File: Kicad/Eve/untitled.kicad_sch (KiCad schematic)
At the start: 9 parts

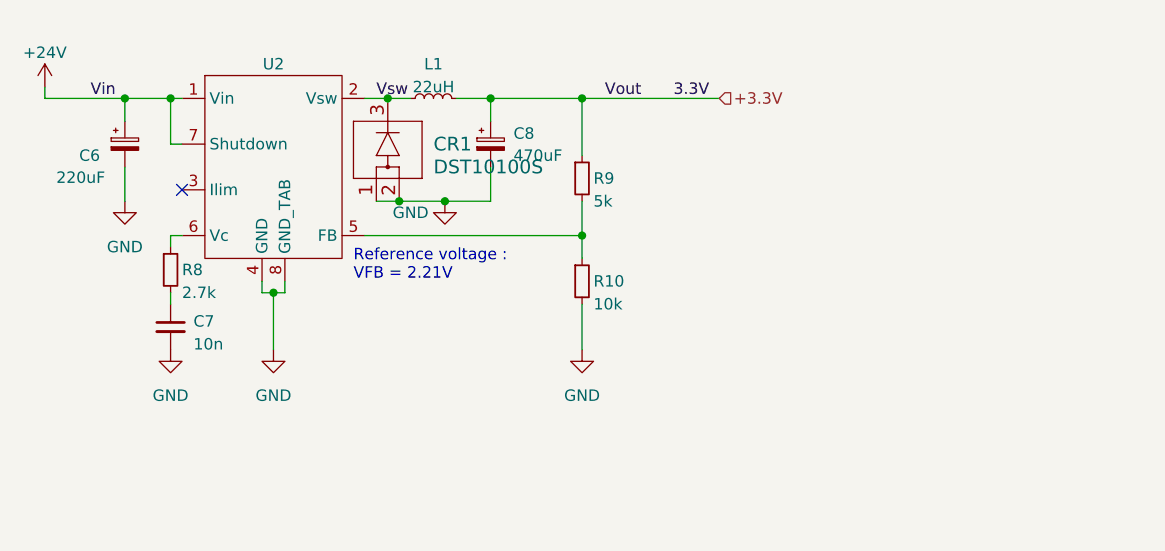
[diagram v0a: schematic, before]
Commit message: updtated Kicad ver 7.11.23
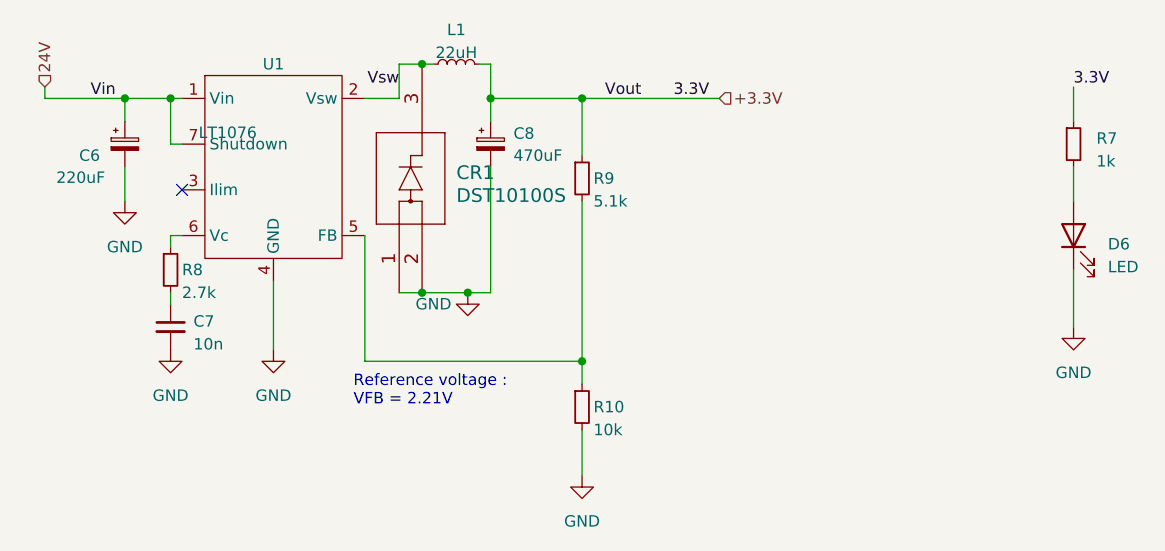
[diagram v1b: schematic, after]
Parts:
- removed U2: ~, libs:LT1076CR-PBF, symbol custom:LT1076
- added D6: LED, LED_SMD:LED_0603_1608Metric_Pad1.05x0.95mm_HandSolder, symbol Device:LED
- added R7: 1k, Resistor_SMD:R_0603_1608Metric_Pad0.98x0.95mm_HandSolder, symbol Device:R_Small
- added U1: LT1076, symbol custom:LT1076
- CR1: footprint libs:DST10100S -> TO277B_LTF
- R9: value 5k -> 5.1k
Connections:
- net +3.3V: now also R7.1
- net GND: now also D6.1 (K), U1.4 (GND)
- net Vsw: now also U1.2 (Vsw)
- net at R8.1: now also U1.6 (Vc)
- net at R10.1, R9.2: now also U1.5 (FB)
- net +24V renamed 24V
- net 24V: now also U1.1 (Vin), U1.7 (Shutdown)
- new net: D6.2 (A), R7.2
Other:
- moved on the sheet: L1, R10
